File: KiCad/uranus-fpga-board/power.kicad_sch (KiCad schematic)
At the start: 0 parts

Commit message: big things happening in JOURNAL
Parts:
- added C86, C87: 10 μF, symbol Device:C_Small
- added C88, C89, C91, C93: 100 nF, symbol Device:C_Small
- added C90, C92: 22 μF, symbol Device:C_Small
- added L1: 2.2 μH, Inductor_SMD:L_Chilisin_BMRA00040415, symbol Device:L
- added R38: 10 kΩ, Resistor_SMD:R_0201_0603Metric, symbol Device:R_Small
- added R39: 4.7 kΩ, Resistor_SMD:R_0402_1005Metric, symbol Device:R_Small
- added R40: 30 kΩ, Resistor_SMD:R_0201_0603Metric, symbol Device:R_Small
- added R41: 52.3 kΩ, Resistor_SMD:R_0402_1005Metric, symbol Device:R_Small
- added R42: 30.9 kΩ, Resistor_SMD:R_0402_1005Metric, symbol Device:R_Small
- added R43: 22.1 kΩ, Resistor_SMD:R_0402_1005Metric, symbol Device:R_Small
- added R44: 13 kΩ, Resistor_SMD:R_0402_1005Metric, symbol Device:R_Small
- added R45: 8.98 kΩ, Resistor_SMD:R_0603_1608Metric, symbol Device:R_Small
- added R46, R47, R48: 200 kΩ, Resistor_SMD:R_0201_0603Metric, symbol Device:R_Small
- added U18: TPS564201DDCR, Package_TO_SOT_SMD:SOT-23-6, symbol Regulator_Switching:TPS565208
- added U19: TMUX1108PWR, Package_SO:TSSOP-16_4.4x5mm_P0.65mm, symbol Analog_Switch:TMUX1108PW
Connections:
- new net: R42.1, U19.6 (S3)
- new net: R45.1, U19.11 (S6)
- new net: R44.1, U19.12 (S5)
- new net: R41.1, U19.5 (S2)
- new net: R43.1, U19.7 (S4)
- new net: R40.2, U18.4 (VFB), U19.8 (D)
- new net: C89.1, L1.1, U18.2 (SW)
- new net: C89.2, U18.6 (VBST)
- new net +12V0: C86.2, C87.2, C88.2, U18.3 (VIN)
- new net +5V0: C93.2, U19.13 (VDD), U19.2 (EN)
- new net GND: C86.1, C87.1, C88.1, C90.1, C91.1, C92.1, C93.1, R38.2, R39.1, R41.2, R42.2, R43.2, R44.2, R45.2, R46.2, R47.1, R48.1, U18.1 (GND), U19.14 (GND), U19.3 (VSS)
- new net VADJ: C90.2, C91.2, C92.2, L1.2, R39.2, R40.1
- new net VADJ_REG_EN: R38.1, U18.5 (EN)
- new net VADJ_SEL_A0: R46.1, U19.1 (A0)
- new net VADJ_SEL_A1: R47.2, U19.16 (A1)
- new net VADJ_SEL_A2: R48.2, U19.15 (A2)
- no-connect marks 0 -> 3
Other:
- note added: "+1V2"
- note added: "+1V5"
- note added: "+1V8"
- note added: "+2V5"
- note added: "+3V3"
- note added: "VADJ Regulator"
- note added: "Ω"
- note added: "μ"

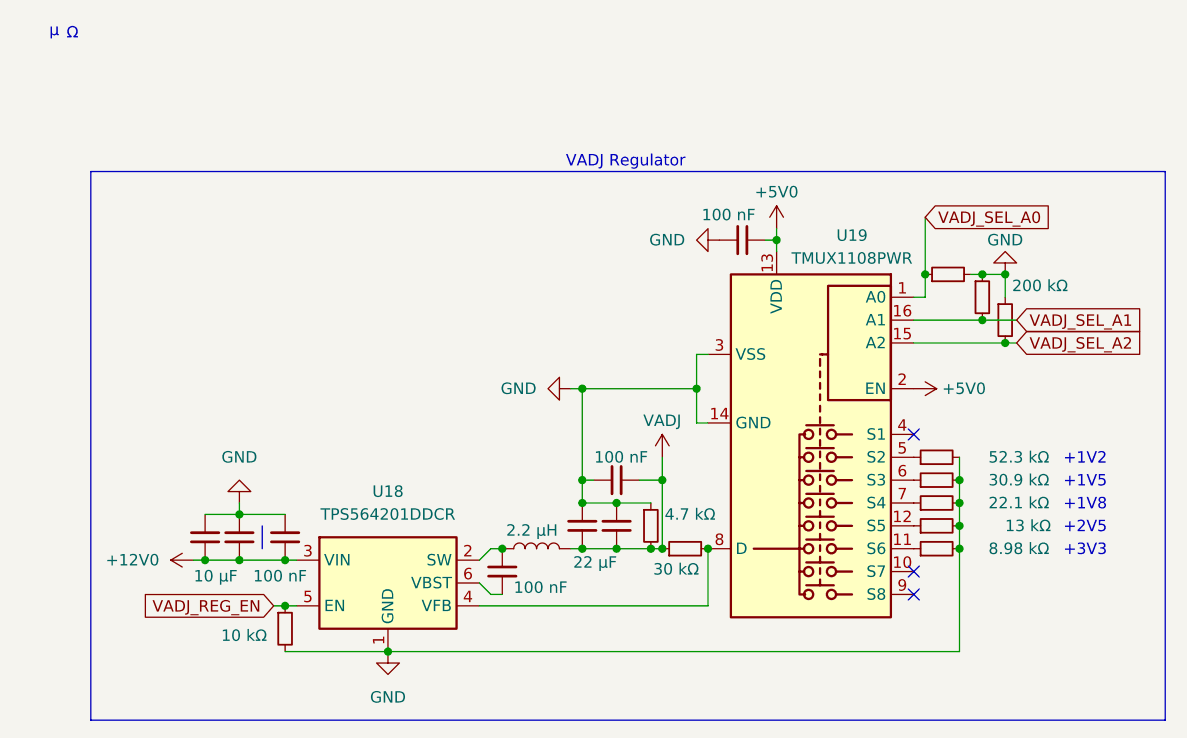
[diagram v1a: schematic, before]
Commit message: big things happening in schematic quality
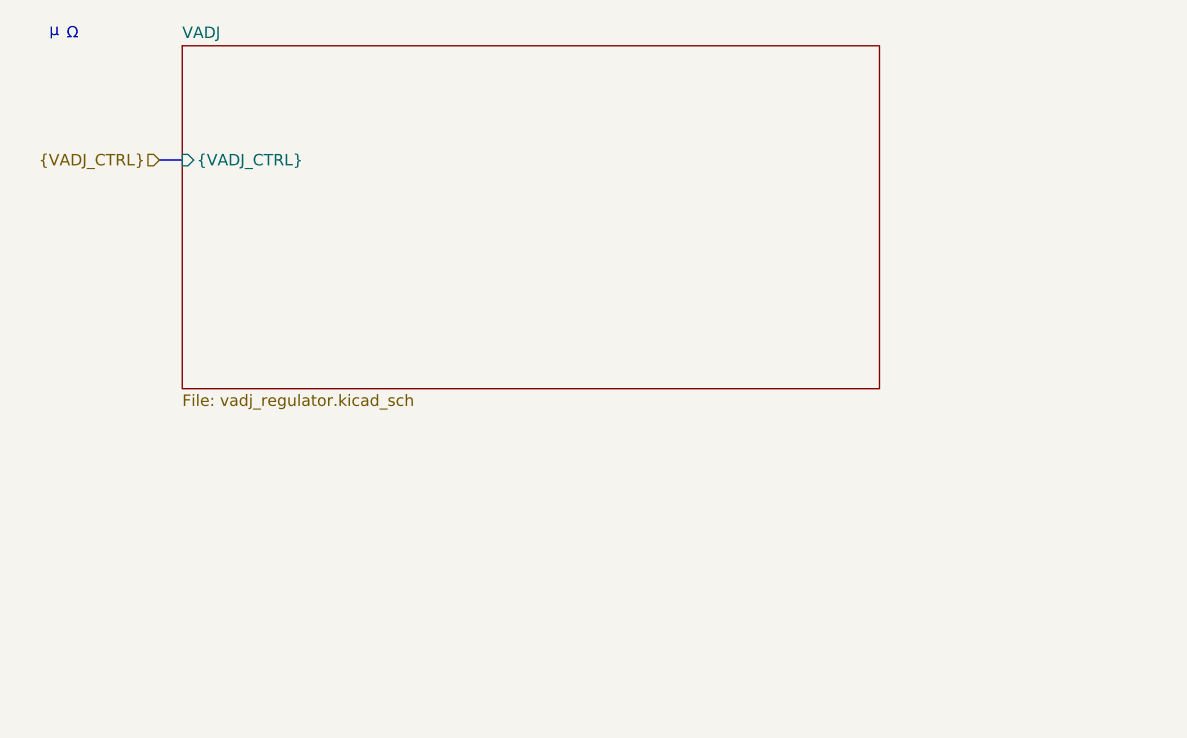
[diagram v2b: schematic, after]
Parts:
- removed C86, C87: 10 μF, symbol Device:C_Small
- removed C88, C89, C91, C93: 100 nF, symbol Device:C_Small
- removed C90, C92: 22 μF, symbol Device:C_Small
- removed L1: 2.2 μH, Inductor_SMD:L_Chilisin_BMRA00040415, symbol Device:L
- removed R38: 10 kΩ, Resistor_SMD:R_0201_0603Metric, symbol Device:R_Small
- removed R39: 4.7 kΩ, Resistor_SMD:R_0402_1005Metric, symbol Device:R_Small
- removed R40: 30 kΩ, Resistor_SMD:R_0201_0603Metric, symbol Device:R_Small
- removed R41: 52.3 kΩ, Resistor_SMD:R_0402_1005Metric, symbol Device:R_Small
- removed R42: 30.9 kΩ, Resistor_SMD:R_0402_1005Metric, symbol Device:R_Small
- removed R43: 22.1 kΩ, Resistor_SMD:R_0402_1005Metric, symbol Device:R_Small
- removed R44: 13 kΩ, Resistor_SMD:R_0402_1005Metric, symbol Device:R_Small
- removed R45: 8.98 kΩ, Resistor_SMD:R_0603_1608Metric, symbol Device:R_Small
- removed R46, R47, R48: 200 kΩ, Resistor_SMD:R_0201_0603Metric, symbol Device:R_Small
- removed U18: TPS564201DDCR, Package_TO_SOT_SMD:SOT-23-6, symbol Regulator_Switching:TPS565208
- removed U19: TMUX1108PWR, Package_SO:TSSOP-16_4.4x5mm_P0.65mm, symbol Analog_Switch:TMUX1108PW
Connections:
- no-connect marks 3 -> 0
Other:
- added sheet VADJ (vadj_regulator.kicad_sch)
- note removed: "+1V2"
- note removed: "+1V5"
- note removed: "+1V8"
- note removed: "+2V5"
- note removed: "+3V3"
- note removed: "VADJ Regulator"
